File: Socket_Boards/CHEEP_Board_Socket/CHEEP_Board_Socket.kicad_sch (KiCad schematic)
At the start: 2 parts

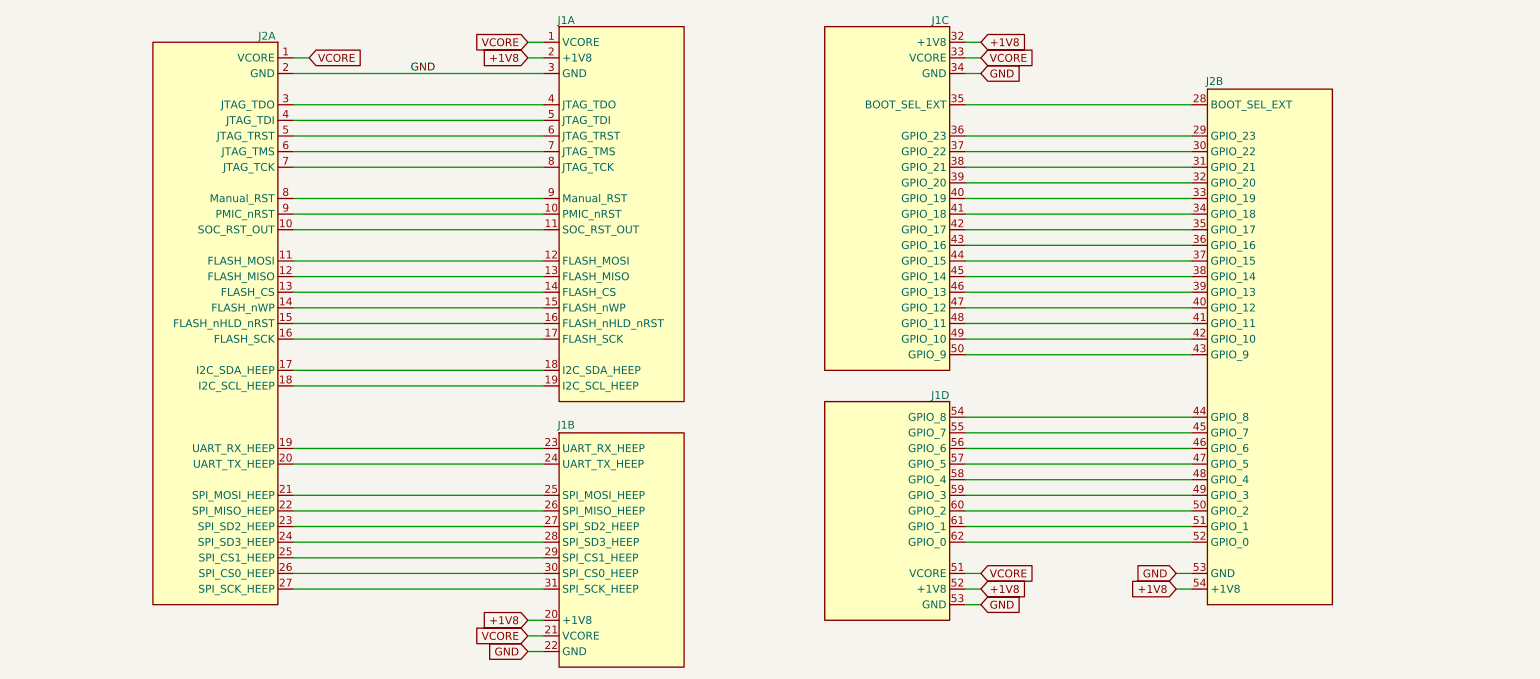
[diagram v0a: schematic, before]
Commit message: Big push. Fixed the issues that were pending. See github
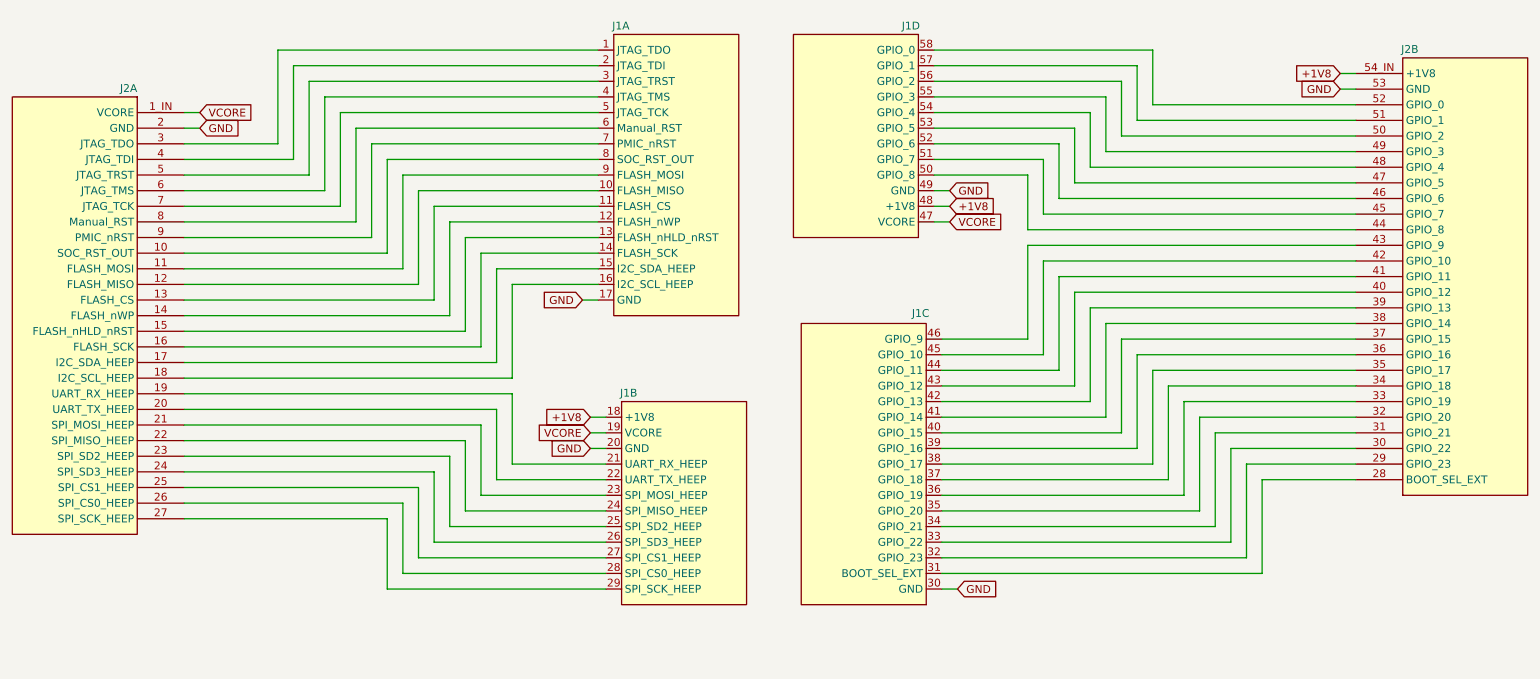
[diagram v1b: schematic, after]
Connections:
- net +1V8: now also J1.18 (+1V8), J1.48 (+1V8), J2.54_IN (+1V8); no longer J1.2 (+1V8), J1.20 (+1V8), J1.32 (+1V8), J1.52 (+1V8), J2.54 (+1V8)
- net GND: now also J1.17 (GND), J1.20 (GND), J1.30 (GND), J1.49 (GND); no longer J1.22 (GND), J1.3 (GND), J1.34 (GND), J1.53 (GND)
- net VCORE: now also J1.19 (VCORE), J1.47 (VCORE), J2.1_IN (VCORE); no longer J1.1 (VCORE), J1.21 (VCORE), J1.33 (VCORE), J1.51 (VCORE), J2.1 (VCORE)
- net at J2.28 (BOOT_SEL_EXT): now also J1.31 (BOOT_SEL_EXT); no longer J1.35 (BOOT_SEL_EXT)
- net at J2.29 (GPIO_23): now also J1.32 (GPIO_23); no longer J1.36 (GPIO_23)
- net at J2.30 (GPIO_22): now also J1.33 (GPIO_22); no longer J1.37 (GPIO_22)
- net at J2.31 (GPIO_21): now also J1.34 (GPIO_21); no longer J1.38 (GPIO_21)
- net at J2.32 (GPIO_20): now also J1.35 (GPIO_20); no longer J1.39 (GPIO_20)
- net at J2.33 (GPIO_19): now also J1.36 (GPIO_19); no longer J1.40 (GPIO_19)
- net at J2.34 (GPIO_18): now also J1.37 (GPIO_18); no longer J1.41 (GPIO_18)
- net at J2.35 (GPIO_17): now also J1.38 (GPIO_17); no longer J1.42 (GPIO_17)
- net at J2.36 (GPIO_16): now also J1.39 (GPIO_16); no longer J1.43 (GPIO_16)
- net at J2.37 (GPIO_15): now also J1.40 (GPIO_15); no longer J1.44 (GPIO_15)
- net at J2.38 (GPIO_14): now also J1.41 (GPIO_14); no longer J1.45 (GPIO_14)
- net at J2.39 (GPIO_13): now also J1.42 (GPIO_13); no longer J1.46 (GPIO_13)
- net at J2.40 (GPIO_12): now also J1.43 (GPIO_12); no longer J1.47 (GPIO_12)
- net at J2.41 (GPIO_11): now also J1.44 (GPIO_11); no longer J1.48 (GPIO_11)
- net at J2.42 (GPIO_10): now also J1.45 (GPIO_10); no longer J1.49 (GPIO_10)
- net at J2.43 (GPIO_9): now also J1.46 (GPIO_9); no longer J1.50 (GPIO_9)
- net at J1.10 (FLASH_MISO): now also J2.12 (FLASH_MISO); no longer J2.9 (PMIC_nRST)
- net at J2.10 (SOC_RST_OUT): now also J1.8 (SOC_RST_OUT); no longer J1.11 (SOC_RST_OUT)
- net at J2.11 (FLASH_MOSI): now also J1.9 (FLASH_MOSI); no longer J1.12 (FLASH_MOSI)
- net at J1.13 (FLASH_nHLD_nRST): now also J2.15 (FLASH_nHLD_nRST); no longer J2.12 (FLASH_MISO)
- net at J2.13 (FLASH_CS): now also J1.11 (FLASH_CS); no longer J1.14 (FLASH_CS)
- net at J2.14 (FLASH_nWP): now also J1.12 (FLASH_nWP); no longer J1.15 (FLASH_nWP)
- net at J1.16 (I2C_SCL_HEEP): now also J2.18 (I2C_SCL_HEEP); no longer J2.15 (FLASH_nHLD_nRST)
- net at J2.16 (FLASH_SCK): now also J1.14 (FLASH_SCK); no longer J1.17 (FLASH_SCK)
- net at J2.17 (I2C_SDA_HEEP): now also J1.15 (I2C_SDA_HEEP); no longer J1.18 (I2C_SDA_HEEP)
- net at J2.3 (JTAG_TDO): now also J1.1 (JTAG_TDO); no longer J1.4 (JTAG_TDO)
- net at J2.4 (JTAG_TDI): now also J1.2 (JTAG_TDI); no longer J1.5 (JTAG_TDI)
- net at J2.5 (JTAG_TRST): now also J1.3 (JTAG_TRST); no longer J1.6 (JTAG_TRST)
- net at J2.6 (JTAG_TMS): now also J1.4 (JTAG_TMS); no longer J1.7 (JTAG_TMS)
- net at J2.7 (JTAG_TCK): now also J1.5 (JTAG_TCK); no longer J1.8 (JTAG_TCK)
- net at J2.8 (Manual_RST): now also J1.6 (Manual_RST); no longer J1.9 (Manual_RST)
- net at J2.44 (GPIO_8): now also J1.50 (GPIO_8); no longer J1.54 (GPIO_8)
- net at J2.45 (GPIO_7): now also J1.51 (GPIO_7); no longer J1.55 (GPIO_7)
- net at J2.46 (GPIO_6): now also J1.52 (GPIO_6); no longer J1.56 (GPIO_6)
- net at J2.47 (GPIO_5): now also J1.53 (GPIO_5); no longer J1.57 (GPIO_5)
- net at J2.48 (GPIO_4): now also J1.54 (GPIO_4); no longer J1.58 (GPIO_4)
- net at J2.49 (GPIO_3): now also J1.55 (GPIO_3); no longer J1.59 (GPIO_3)
- net at J2.50 (GPIO_2): now also J1.56 (GPIO_2); no longer J1.60 (GPIO_2)
- net at J2.51 (GPIO_1): now also J1.57 (GPIO_1); no longer J1.61 (GPIO_1)
- net at J2.52 (GPIO_0): now also J1.58 (GPIO_0); no longer J1.62 (GPIO_0)
- net at J2.19 (UART_RX_HEEP): now also J1.21 (UART_RX_HEEP); no longer J1.23 (UART_RX_HEEP)
- net at J2.20 (UART_TX_HEEP): now also J1.22 (UART_TX_HEEP); no longer J1.24 (UART_TX_HEEP)
- net at J2.21 (SPI_MOSI_HEEP): now also J1.23 (SPI_MOSI_HEEP); no longer J1.25 (SPI_MOSI_HEEP)
- net at J2.22 (SPI_MISO_HEEP): now also J1.24 (SPI_MISO_HEEP); no longer J1.26 (SPI_MISO_HEEP)
- net at J2.23 (SPI_SD2_HEEP): now also J1.25 (SPI_SD2_HEEP); no longer J1.27 (SPI_SD2_HEEP)
- net at J2.24 (SPI_SD3_HEEP): now also J1.26 (SPI_SD3_HEEP); no longer J1.28 (SPI_SD3_HEEP)
- net at J2.25 (SPI_CS1_HEEP): now also J1.27 (SPI_CS1_HEEP); no longer J1.29 (SPI_CS1_HEEP)
- net at J2.26 (SPI_CS0_HEEP): now also J1.28 (SPI_CS0_HEEP); no longer J1.30 (SPI_CS0_HEEP)
- net at J2.27 (SPI_SCK_HEEP): now also J1.29 (SPI_SCK_HEEP); no longer J1.31 (SPI_SCK_HEEP)
- new net: J1.7 (PMIC_nRST), J2.9 (PMIC_nRST)
